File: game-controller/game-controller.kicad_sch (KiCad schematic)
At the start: 22 parts, among them SW1 TS-1187A-B-A-B, SW2 TS-1187A-B-A-B, SW3 TS-1187A-B-A-B, SW4 TS-1187A-B-A-B, SW5 TS-1187A-B-A-B, SW6 TS-1187A-B-A-B, SW7 TS-1187A-B-A-B, SW8 TS-1187A-B-A-B, U1 STM32F103C8T6, X1 TAXM8M4RDBCCT2T

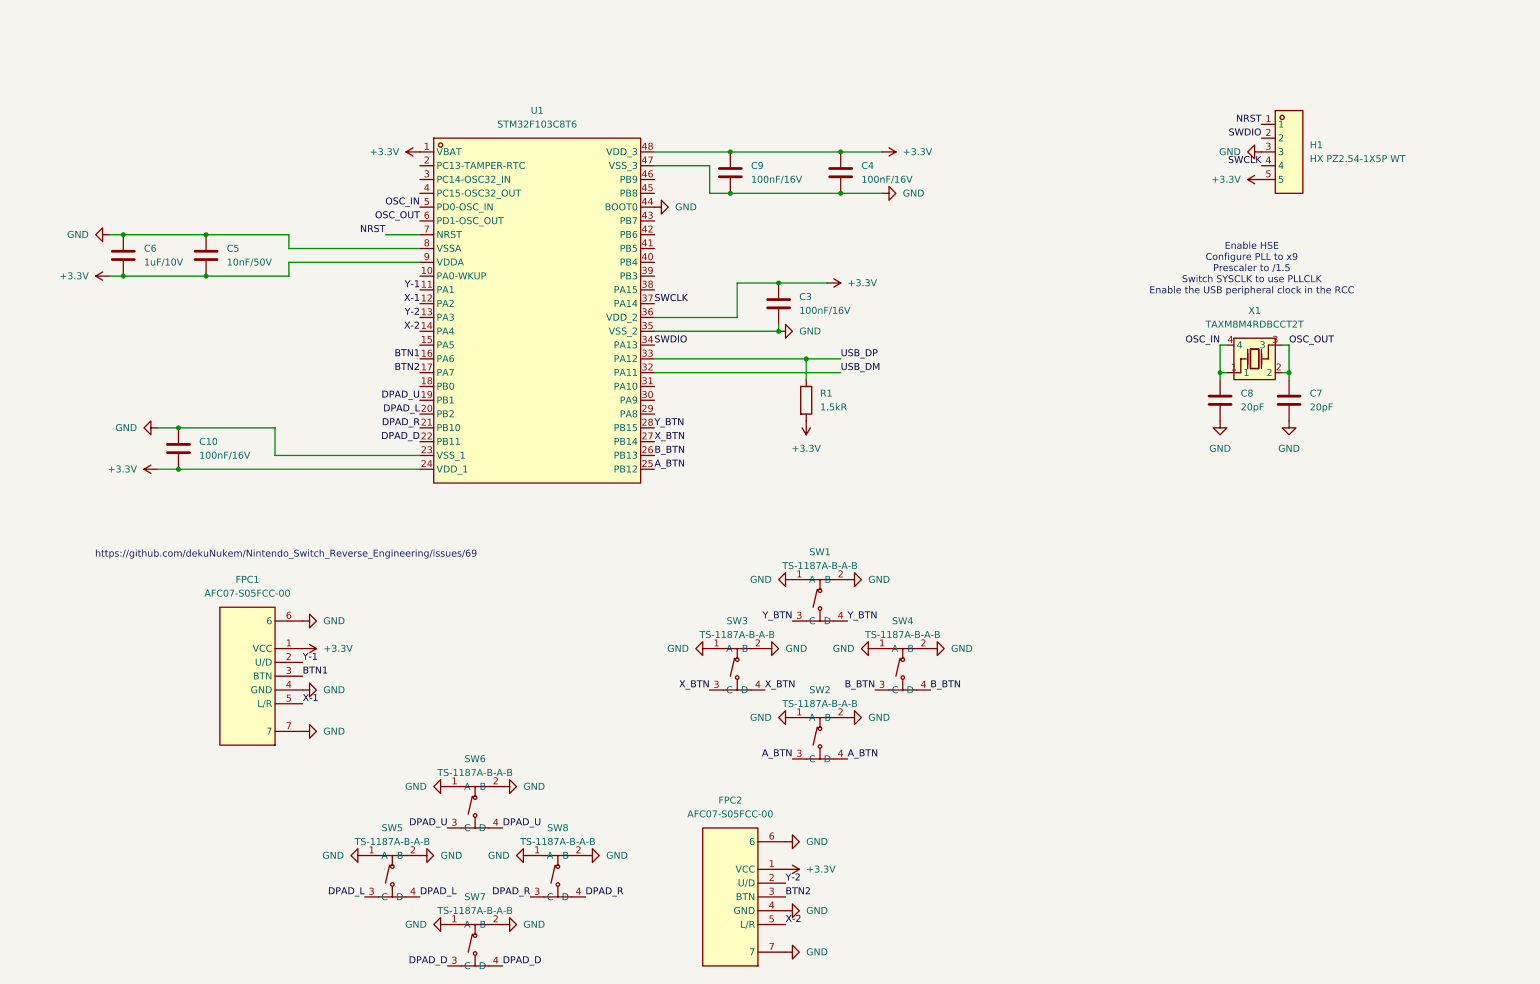
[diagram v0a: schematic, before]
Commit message: Schematics pretty solid now, need to check it again later
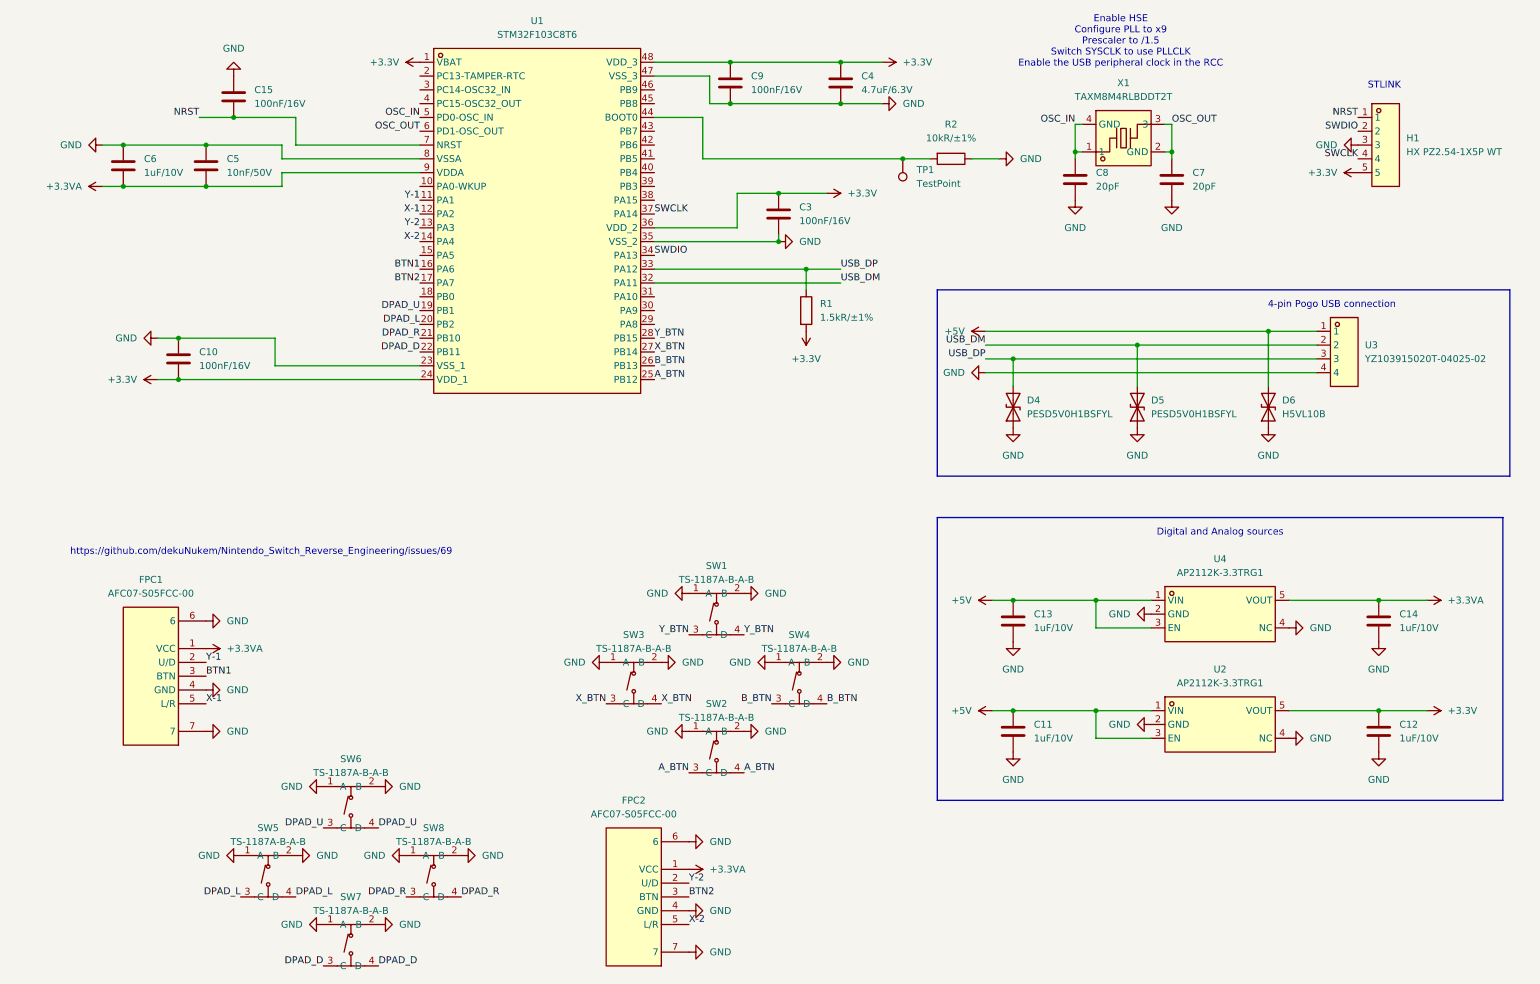
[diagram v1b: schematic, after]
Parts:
- removed X1: TAXM8M4RDBCCT2T, parts:CRYSTAL-SMD_4P-L3.2-W2.5-BL, symbol parts:TAXM8M4RDBCCT2T
- added C11, C12, C13, C14: 1uF/10V, Capacitor_SMD:C_0402_1005Metric, symbol Device:C
- added C15: 100nF/16V, Capacitor_SMD:C_0402_1005Metric, symbol Device:C
- added D4, D5: PESD5V0H1BSFYL, Diode_SMD:Nexperia_DSN0603-2_0.6x0.3mm_P0.4mm, symbol Device:D_TVS
- added D6: H5VL10B, Diode_SMD:D_SOD-882, symbol Device:D_TVS
- added R2: 10kR/±1%, Resistor_SMD:R_0402_1005Metric, symbol Device:R
- added TP1: TestPoint, TestPoint:TestPoint_Pad_1.5x1.5mm, symbol Connector:TestPoint
- added U2, U4: AP2112K-3.3TRG1, parts:SOT-25-5_L2.9-W1.6-P0.95-LS2.8-BL, symbol parts:AP2112K-3.3TRG1
- added U3: YZ103915020T-04025-02, parts:CONN-SMD_YZ103915020T-04025-01, symbol parts:YZ103915020T-04025-02
- added X1: TAXM8M4RLBDDT2T, parts:CRYSTAL-SMD_4P-L3.2-W2.5-BL, symbol parts:TAXM8M4RLBDDT2T
- C4: value 100nF/16V -> 4.7uF/6.3V; LCSC Part C328914 -> C380302
- R1: value 1.5kR -> 1.5kR/±1%
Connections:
- net +3.3V: now also C12.1, U2.5 (VOUT); no longer C5.2, C6.2, FPC1.1 (VCC), FPC2.1 (VCC), U1.9 (VDDA)
- net GND: now also C11.2, C12.2, C13.2, C14.2, C15.1, D4.1 (A1), D5.1 (A1), D6.1 (A1), R2.1, U2.2 (GND), U2.4 (NC), U3.4, U4.2 (GND), U4.4 (NC); no longer U1.44 (BOOT0)
- net NRST: now also C15.2
- net OSC_IN: now also X1.1, X1.4 (GND)
- net OSC_OUT: now also X1.2 (GND), X1.3
- net USB_DM: now also D5.2 (A2), U3.2
- net USB_DP: now also D4.2 (A2), U3.3
- new net: R2.2, TP1.1, U1.44 (BOOT0)
- new net +3.3VA: C14.1, C5.2, C6.2, FPC1.1 (VCC), FPC2.1 (VCC), U1.9 (VDDA), U4.5 (VOUT)
- new net +5V: C11.1, C13.1, D6.2 (A2), U2.1 (VIN), U2.3 (EN), U3.1, U4.1 (VIN), U4.3 (EN)
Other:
- note added: "4-pin Pogo USB connection"
- note added: "Digital and Analog sources"
- note added: "STLINK"
- moved on the sheet: C10, C3, C4, C5, C6, C7, C8, C9, FPC1, FPC2, H1, R1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
